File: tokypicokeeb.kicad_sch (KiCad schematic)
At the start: 129 parts, among them SW1 SW_Push, U1 PicoW

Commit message: 1/2 diodes
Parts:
- D1, D10, D11, D12, D13, D14, D15, D16, D17, D18, D19, D2, D20, D21, D22, D23, D24, D25, D26, D27, D28, D29, D3, D30, D31, D32, D33, D34, D35, D36, D37, D38, D39, D4, D40, D41, D42, D43, D44, D45, D46, D47, D48, D49, D5, D50, D51, D52, D53, D54, D55, D56, D57, D58, D59, D6, D60, D61, D62, D63, D7, D8, D9: footprint random-keyboard-parts:D_SOD-123-Pretty -> ScottoKeebs_Components:Diode_DO-35

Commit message: finished the diodes placement
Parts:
- D1, D10, D11, D12, D13, D14, D15, D16, D17, D18, D19, D2, D20, D21, D22, D23, D24, D25, D26, D27, D28, D29, D3, D30, D31, D32, D33, D34, D35, D36, D37, D38, D39, D4, D40, D41, D42, D43, D44, D45, D46, D47, D48, D49, D5, D50, D51, D52, D53, D54, D55, D56, D57, D58, D59, D6, D60, D61, D62, D63, D7, D8, D9: footprint ScottoKeebs_Components:Diode_DO-35 -> random-keyboard-parts:D_SOD-123-Pretty

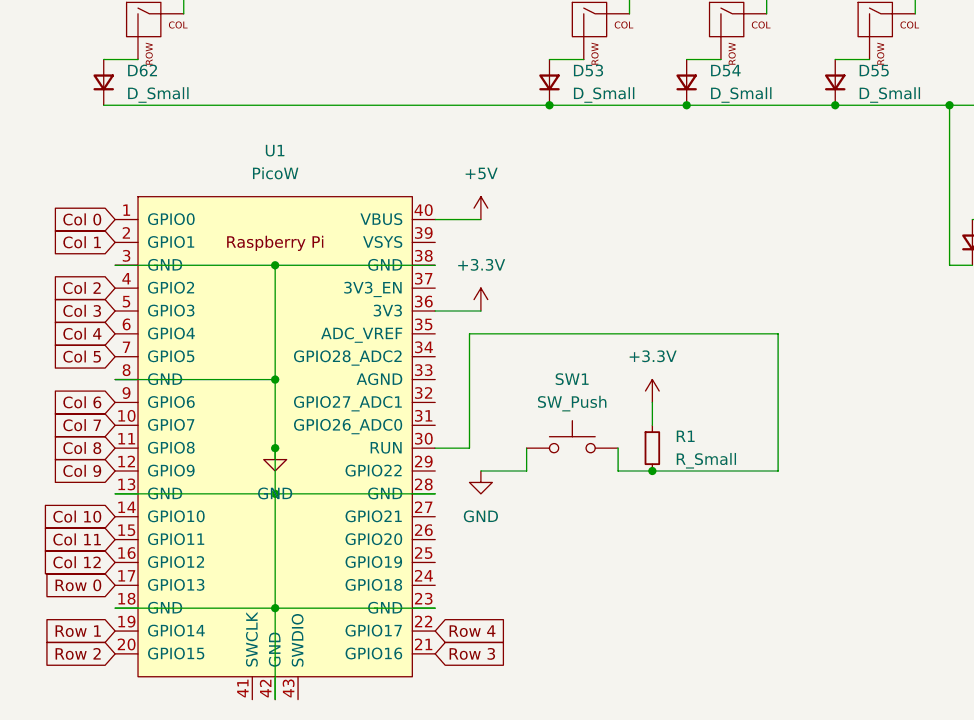
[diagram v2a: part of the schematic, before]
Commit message: finished ver. 1
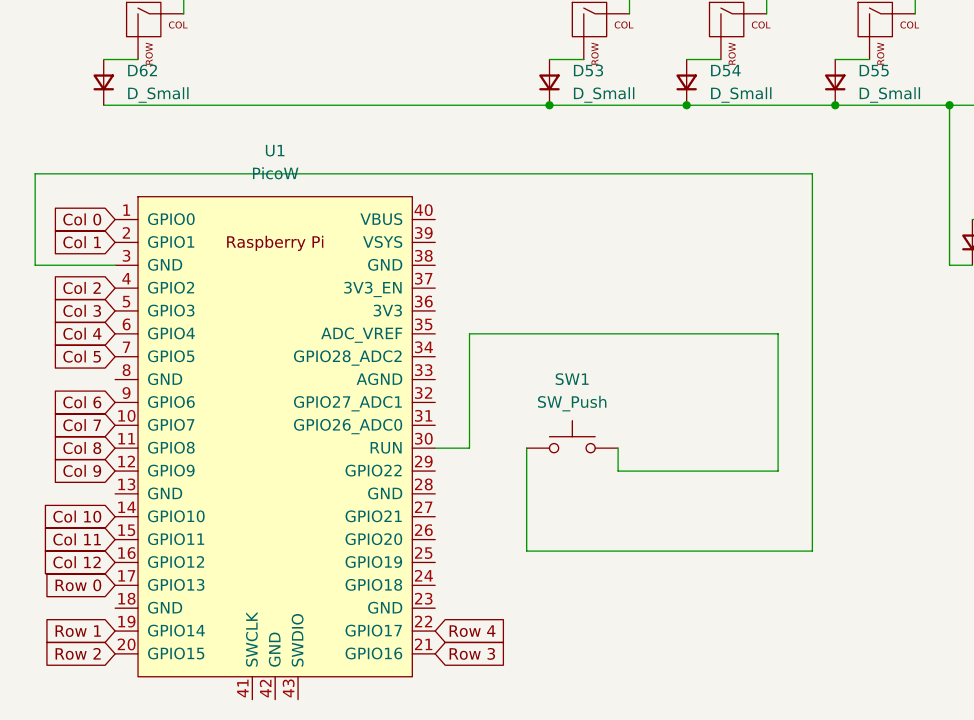
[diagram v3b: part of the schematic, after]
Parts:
- removed R1: R_Small, Resistor_SMD:R_0805_2012Metric, symbol Device:R_Small
- D1, D10, D11, D12, D13, D14, D15, D16, D17, D18, D19, D2, D20, D21, D22, D23, D24, D25, D26, D27, D28, D29, D3, D30, D31, D32, D33, D34, D35, D36, D37, D38, D39, D4, D40, D41, D42, D43, D44, D45, D46, D47, D48, D49, D5, D50, D51, D52, D53, D54, D55, D56, D57, D58, D59, D6, D60, D61, D62, D63, D7, D8, D9: footprint random-keyboard-parts:D_SOD-123-Pretty -> ScottoKeebs_Components:Diode_DO-35
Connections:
- net +3.3V: no longer names the net of U1.36 (3V3)
- net +5V: no longer names the net of U1.40 (VBUS)
- removed net GND: SW1.1, U1.13 (GND), U1.18 (GND), U1.23 (GND), U1.28 (GND), U1.3 (GND), U1.38 (GND), U1.42 (GND), U1.8 (GND)
- new net: SW1.1, U1.3 (GND)
